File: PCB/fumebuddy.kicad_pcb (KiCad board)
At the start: 2 copper layers, 26.2 x 67.2 mm, 23 parts, among them J1 USB_B_Micro, J2 STATION, J3 esp32buddy, J4 TOUCH, SW1 SW_SPDT, SW2 SW_SPDT, U1 AP7361C-33E, U2 CPC1017N (NO), U4 ESP32-WROOM-32D, U5 CPC1117N (NC)

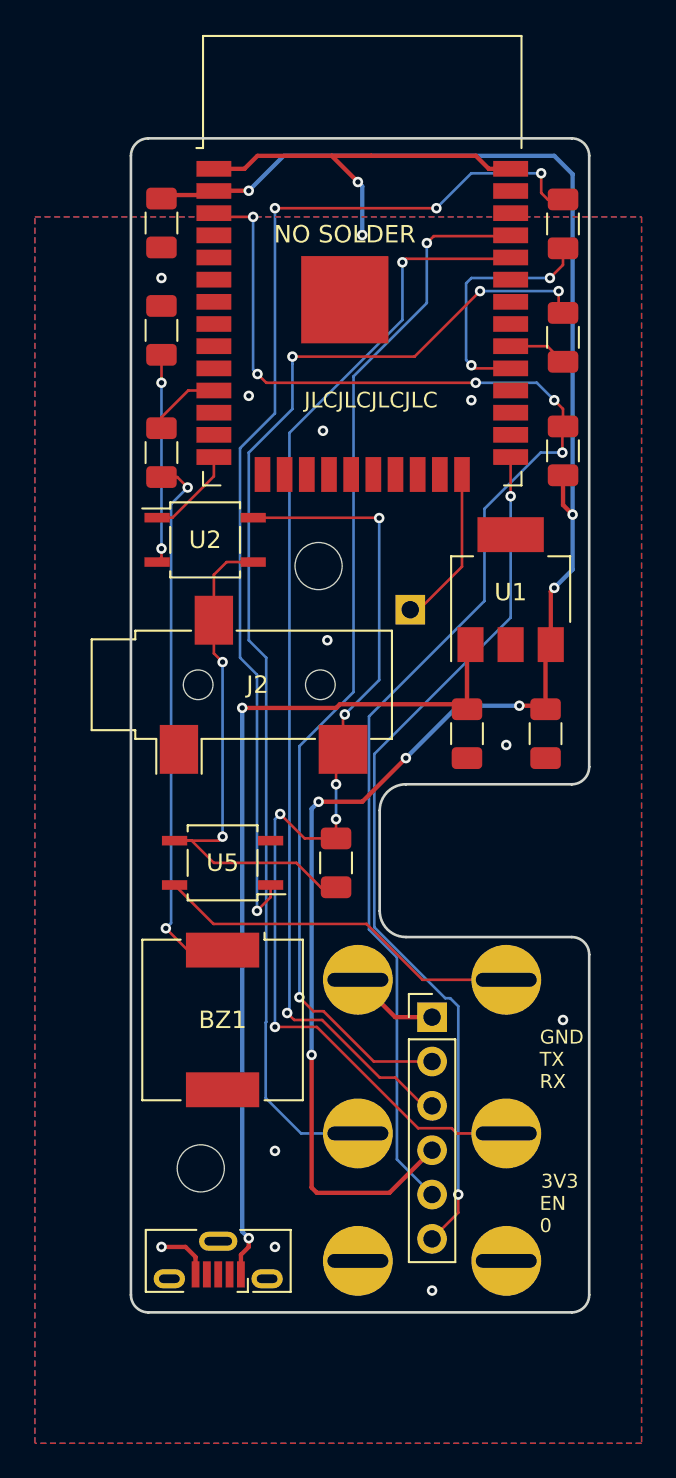
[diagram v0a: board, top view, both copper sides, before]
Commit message: updates
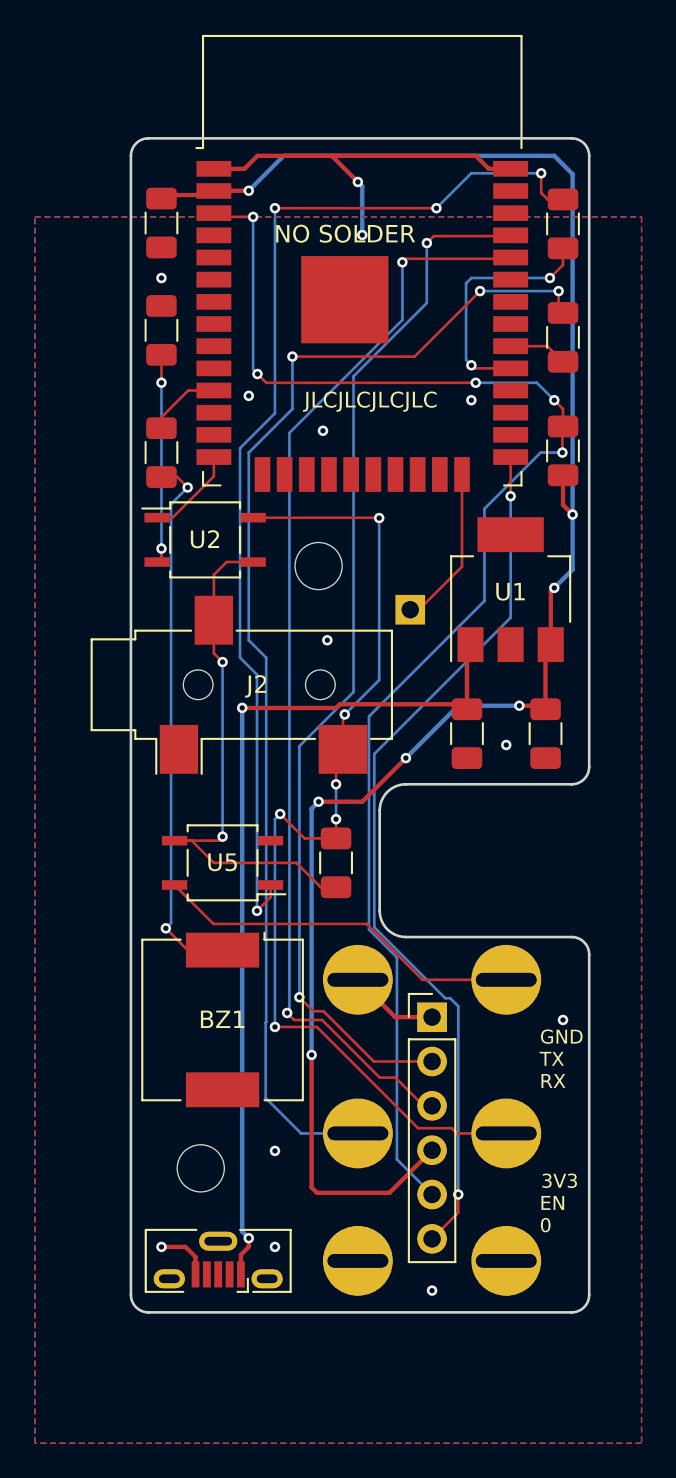
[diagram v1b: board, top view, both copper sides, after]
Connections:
- J1 pad 2: (no net) -> unconnected-(J1-D--Pad2)
- J1 pad 3: (no net) -> unconnected-(J1-D+-Pad3)
- J1 pad 4: (no net) -> unconnected-(J1-ID-Pad4)
- J1 pad 6: Net-(J1-Pad6) -> unconnected-(J1-Shield-Pad6)
- J2 pad S: (no net) -> unconnected-(J2-PadS)
- SW1 pad 3: (no net) -> unconnected-(SW1-C-Pad3)
- SW2 pad 3: (no net) -> unconnected-(SW2-C-Pad3)
- U4 pad 10: (no net) -> unconnected-(U4-IO25-Pad10)
- U4 pad 12: (no net) -> unconnected-(U4-IO27-Pad12)
- U4 pad 13: (no net) -> unconnected-(U4-IO14-Pad13)
- U4 pad 16: (no net) -> unconnected-(U4-IO13-Pad16)
- U4 pad 17: (no net) -> unconnected-(U4-SHD/SD2-Pad17)
- U4 pad 18: (no net) -> unconnected-(U4-SWP/SD3-Pad18)
- U4 pad 19: (no net) -> unconnected-(U4-SCS/CMD-Pad19)
- U4 pad 20: (no net) -> unconnected-(U4-SCK/CLK-Pad20)
- U4 pad 21: (no net) -> unconnected-(U4-SDO/SD0-Pad21)
- U4 pad 22: (no net) -> unconnected-(U4-SDI/SD1-Pad22)
- U4 pad 23: (no net) -> unconnected-(U4-IO15-Pad23)
- U4 pad 26: (no net) -> unconnected-(U4-IO4-Pad26)
- U4 pad 27: (no net) -> unconnected-(U4-IO16-Pad27)
- U4 pad 28: (no net) -> unconnected-(U4-IO17-Pad28)
- U4 pad 31: (no net) -> unconnected-(U4-IO19-Pad31)
- U4 pad 32: (no net) -> unconnected-(U4-NC-Pad32)
- U4 pad 33: (no net) -> unconnected-(U4-IO21-Pad33)
- U4 pad 36: (no net) -> unconnected-(U4-IO22-Pad36)
- U4 pad 37: (no net) -> unconnected-(U4-IO23-Pad37)
- U4 pad 4: (no net) -> unconnected-(U4-SENSOR_VP-Pad4)
- U4 pad 5: (no net) -> unconnected-(U4-SENSOR_VN-Pad5)
- U4 pad 6: (no net) -> unconnected-(U4-IO34-Pad6)
- U4 pad 7: (no net) -> unconnected-(U4-IO35-Pad7)
- U4 pad 8: (no net) -> unconnected-(U4-IO32-Pad8)
- U4 pad 9: (no net) -> unconnected-(U4-IO33-Pad9)
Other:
- net class Default removed
- net class Power removed
